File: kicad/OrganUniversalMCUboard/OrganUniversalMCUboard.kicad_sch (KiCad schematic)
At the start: 25 parts, among them J11 GPIO, J7 I2S, J8 SPI, J9 I2C, SW1 MODES, U1 ESP32-S3-DevKitC

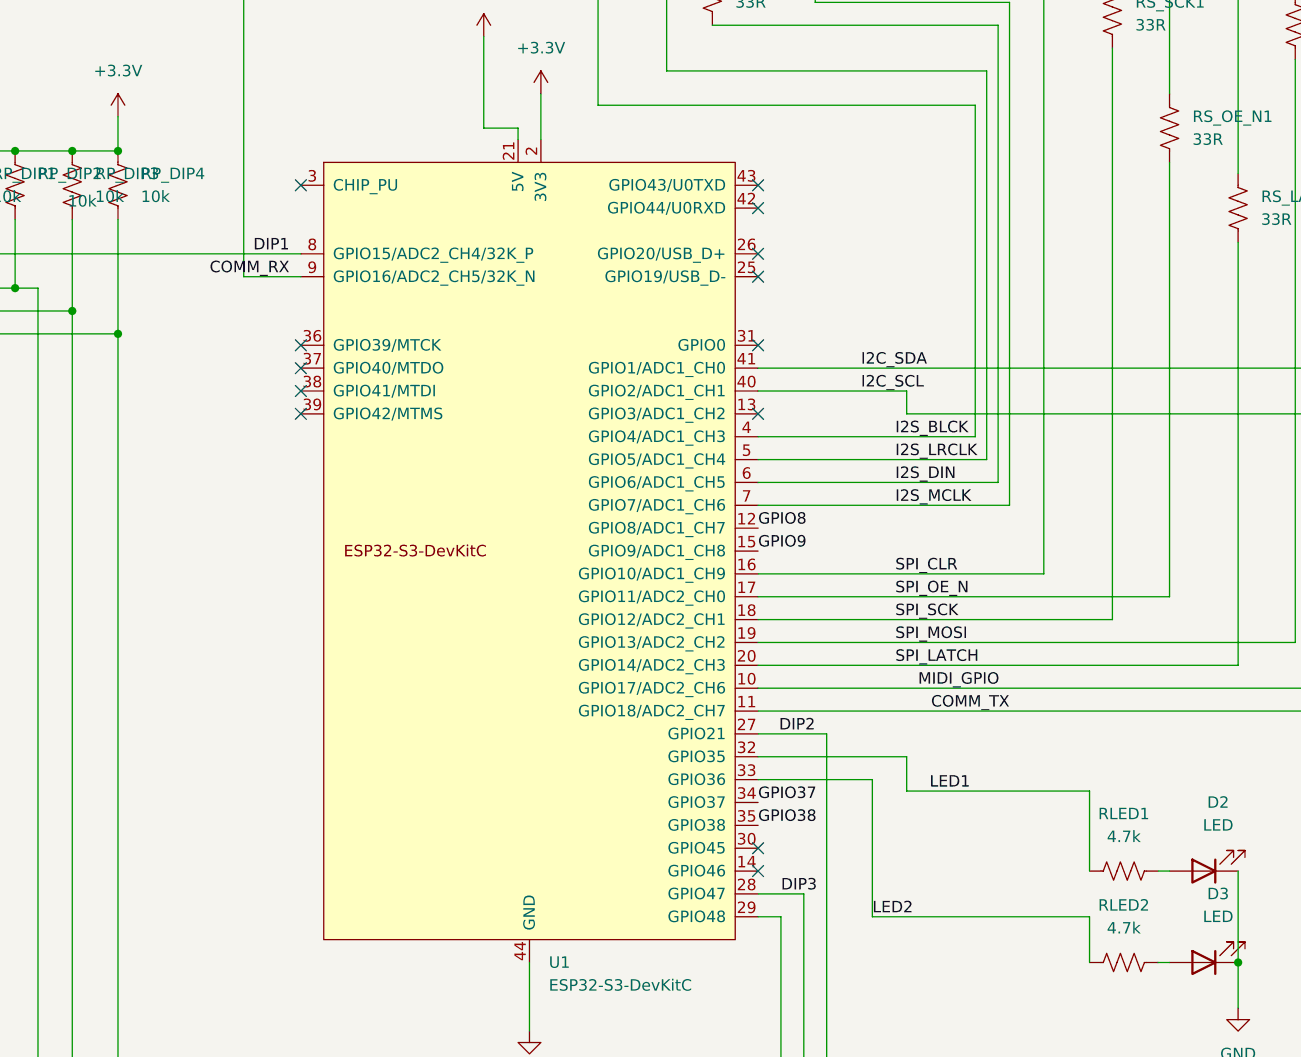
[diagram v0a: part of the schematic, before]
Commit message: Something...
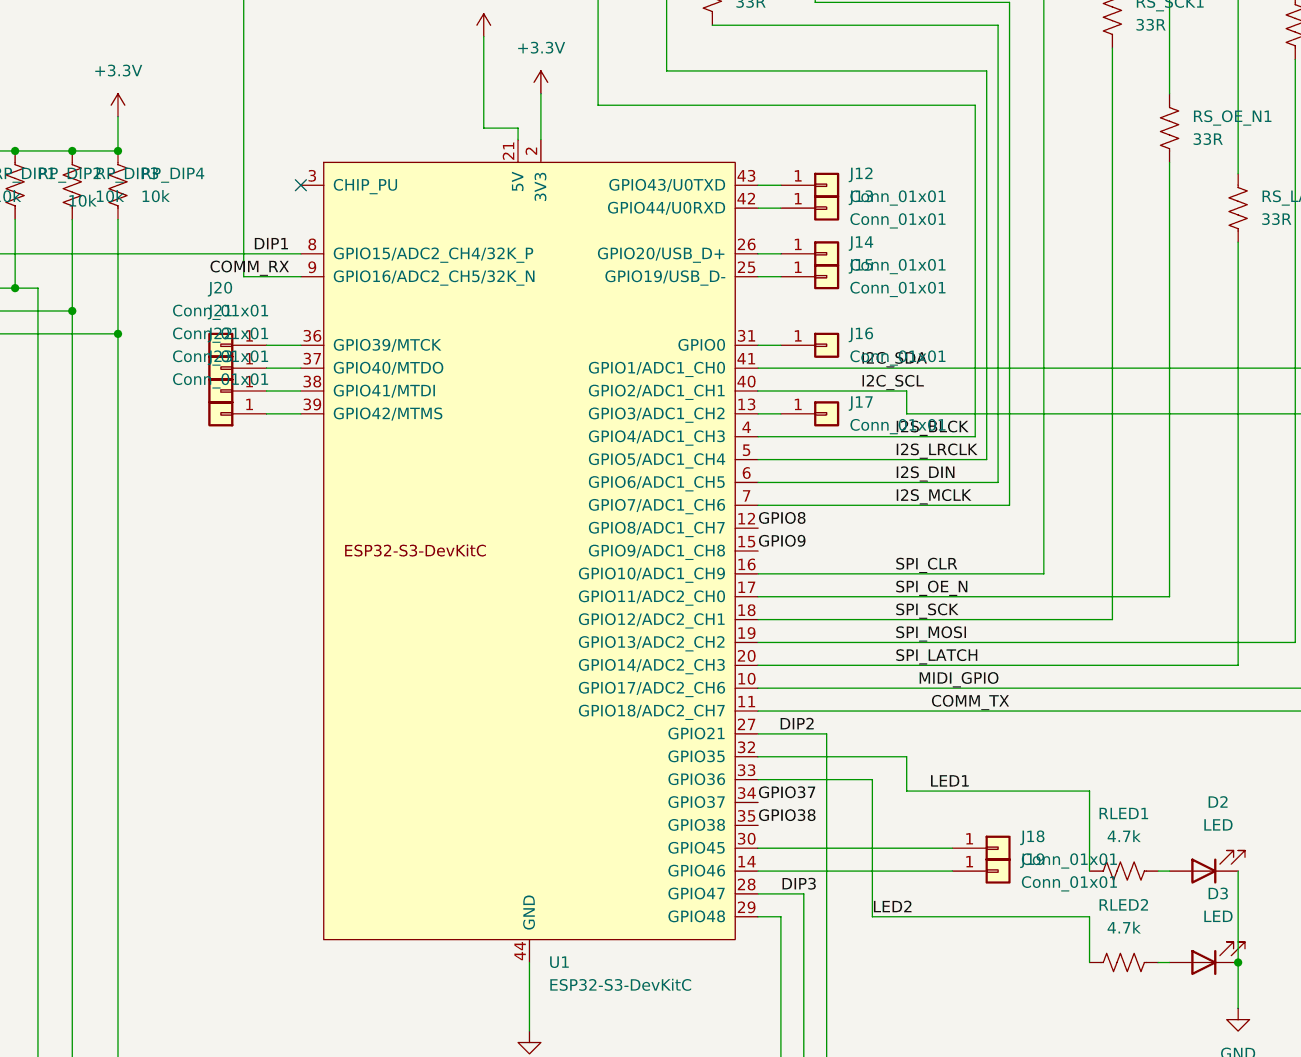
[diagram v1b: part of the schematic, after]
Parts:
- added J12, J13, J14, J15, J16, J17, J18, J19, J20, J21, J22, J23: Conn_01x01, Connector_PinHeader_2.54mm:PinHeader_1x01_P2.54mm_Vertical, symbol Connector_Generic:Conn_01x01
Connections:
- net at U1.13 (GPIO3/ADC1_CH2): now also J17.1 (Pin_1)
- net at U1.14 (GPIO46): now also J19.1 (Pin_1)
- net at U1.25 (GPIO19/USB_D-): now also J15.1 (Pin_1)
- net at U1.26 (GPIO20/USB_D+): now also J14.1 (Pin_1)
- net at U1.30 (GPIO45): now also J18.1 (Pin_1)
- net at U1.31 (GPIO0): now also J16.1 (Pin_1)
- net at U1.36 (GPIO39/MTCK): now also J20.1 (Pin_1)
- net at U1.37 (GPIO40/MTDO): now also J21.1 (Pin_1)
- net at U1.38 (GPIO41/MTDI): now also J22.1 (Pin_1)
- net at U1.39 (GPIO42/MTMS): now also J23.1 (Pin_1)
- net at U1.42 (GPIO44/U0RXD): now also J13.1 (Pin_1)
- net at U1.43 (GPIO43/U0TXD): now also J12.1 (Pin_1)
- no-connect marks 14 -> 2
